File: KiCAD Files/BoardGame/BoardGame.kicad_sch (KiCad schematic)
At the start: 0 parts

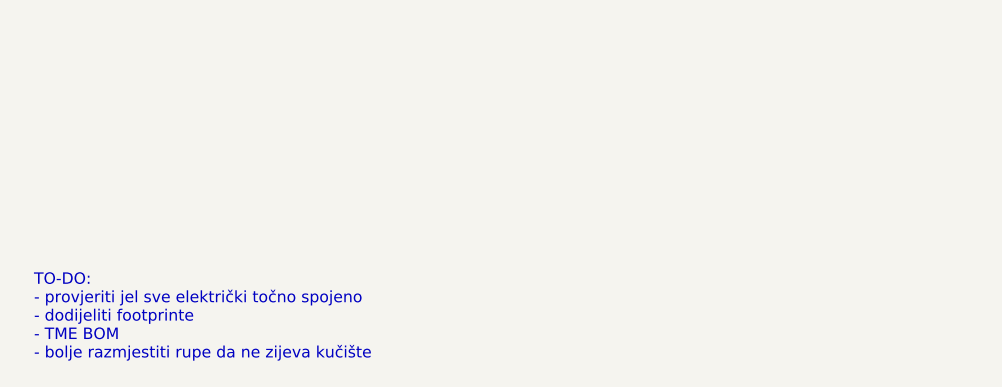
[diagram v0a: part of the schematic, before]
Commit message: update
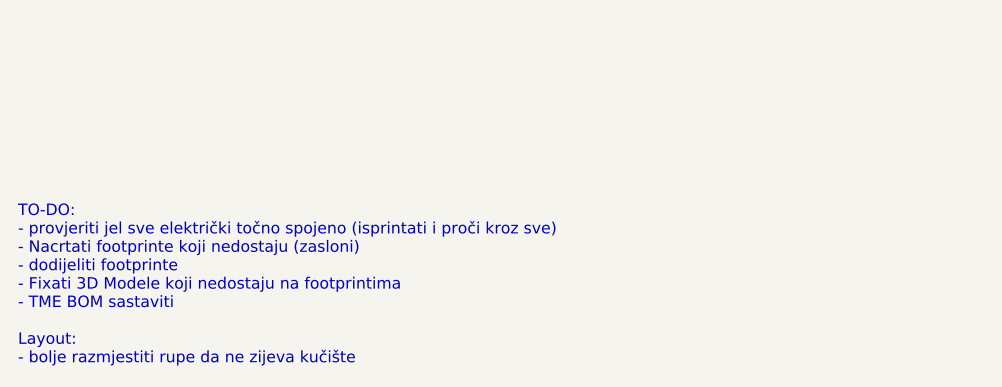
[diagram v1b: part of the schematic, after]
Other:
- note added: "TO-DO: - provjeriti jel sve električki točno spojeno (isprintati i proči kroz sve) - Nacrtati footprinte koji nedostaju (zasloni) - dodijeliti footprinte - Fixati 3D Modele koji nedostaju na footprintima - TME BOM sastaviti Layout: - bolje razmjestiti rupe da ne zijeva kučište"
- note removed: "TO-DO: - provjeriti jel sve električki točno spojeno - dodijeliti footprinte - TME BOM - bolje razmjestiti rupe da ne zijeva kučište"
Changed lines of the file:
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@@
 		)
 	)
-	(text "TO-DO:\n- provjeriti jel sve električki točno spojeno\n- dodijeliti footprinte\n- TME BOM\n- bolje razmjestiti rupe da ne zijeva kučište"
+	(text "TO-DO:\n- provjeriti jel sve električki točno spojeno (isprintati i proči kroz sve)\n- Nacrtati footprinte koji nedostaju (zasloni)\n- dodijeliti footprinte\n- Fixati 3D Modele koji nedostaju na footprintima\n- TME BOM sastaviti\n\nLayout:\n- bolje razmjestiti rupe da ne zijeva kučište"
 		(exclude_from_sim no)
-		(at 17.78 188.214 0)
+		(at 16.002 184.658 0)
 		(effects
 			(font
